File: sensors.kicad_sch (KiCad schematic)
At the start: 3 parts, among them J1 Conn_Coaxial, U2 MAX-M8C

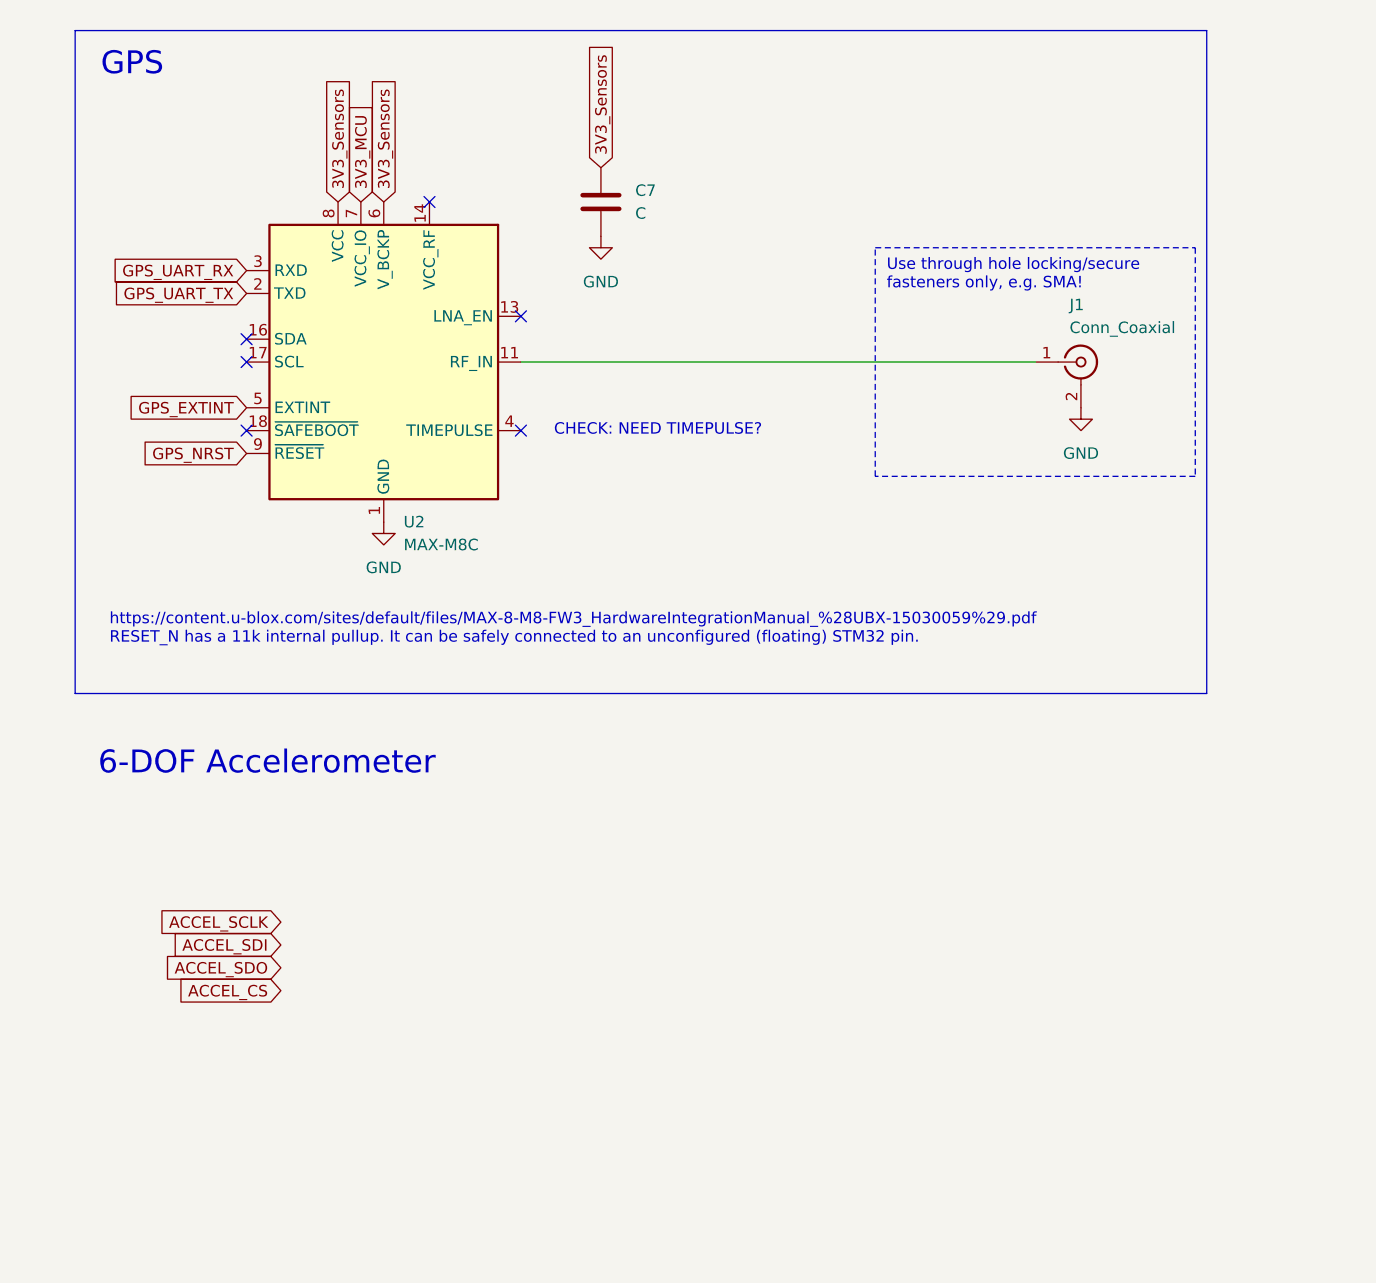
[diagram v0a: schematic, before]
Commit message: Power Supply Speccing, IMU, Eyeballs
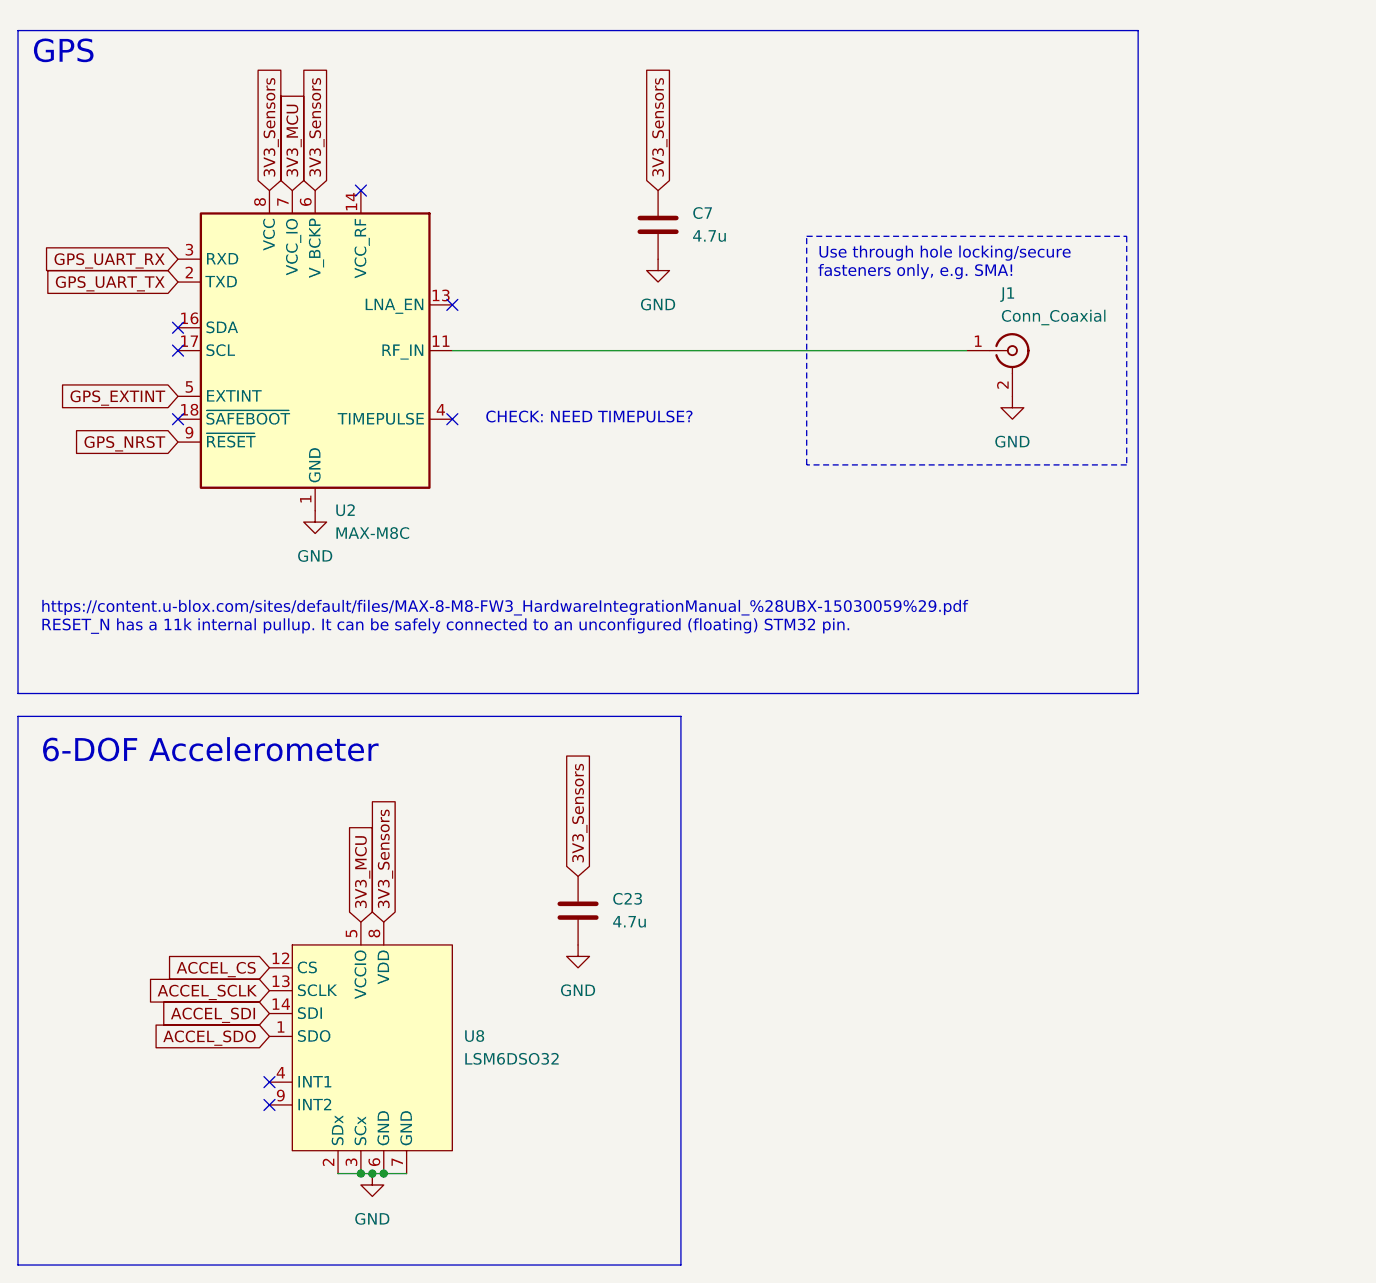
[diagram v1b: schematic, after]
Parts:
- added C23: 4.7u, Capacitor_SMD:C_0805_2012Metric, symbol Device:C
- added U8: LSM6DSO32, Package_LGA:LGA-14_3x2.5mm_P0.5mm_LayoutBorder3x4y, symbol 0_airbrake_symbols:LSM6DSO32
- C7: value C -> 4.7u
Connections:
- net 3V3_MCU: now also U8.5 (VCCIO)
- net 3V3_Sensors: now also C23.1, U8.8 (VDD)
- net ACCEL_CS: now also U8.12 (CS)
- net ACCEL_SCLK: now also U8.13 (SCLK)
- net ACCEL_SDI: now also U8.14 (SDI)
- net ACCEL_SDO: now also U8.1 (SDO)
- net GND: now also C23.2, U8.2 (SDx), U8.3 (SCx), U8.6 (GND), U8.7 (GND)
- no-connect marks 6 -> 8
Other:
- moved on the sheet: J1, U2
